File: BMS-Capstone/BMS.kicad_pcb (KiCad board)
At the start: 2 copper layers, 16 parts, among them IC1 MP2643, Q1 FODM121, Q2 FODM121

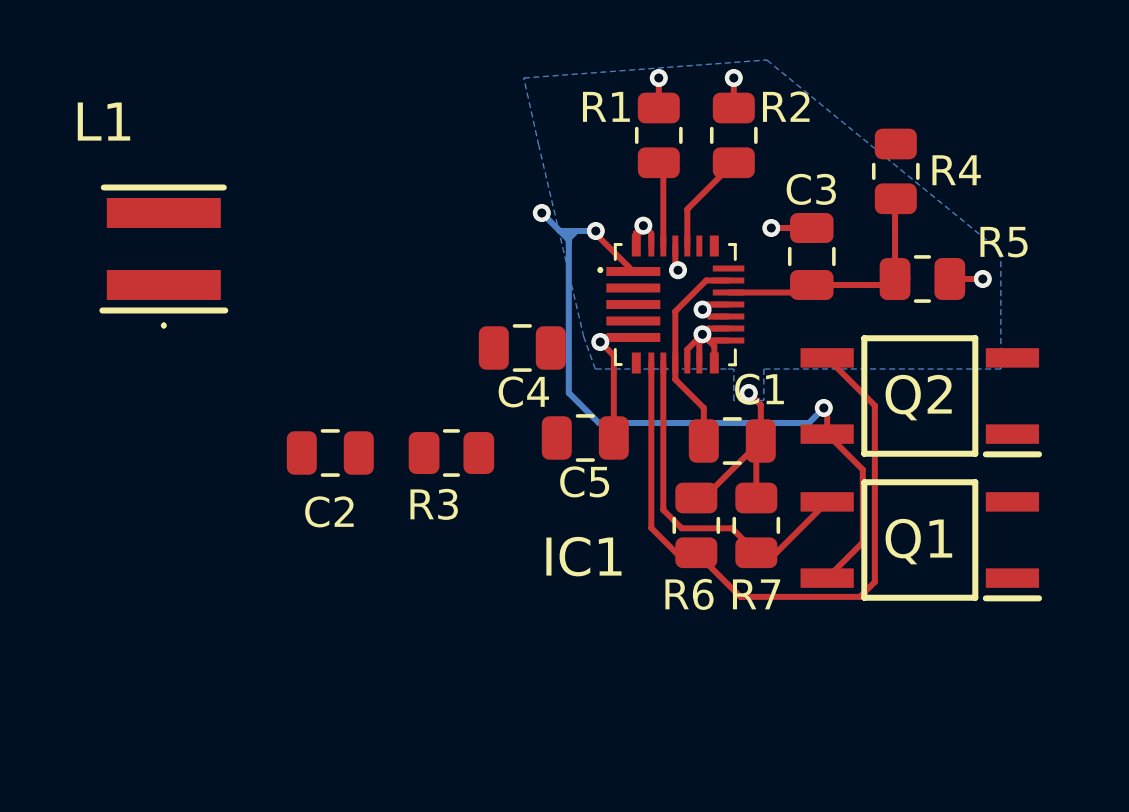
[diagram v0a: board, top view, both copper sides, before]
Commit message: Redid the whole thing
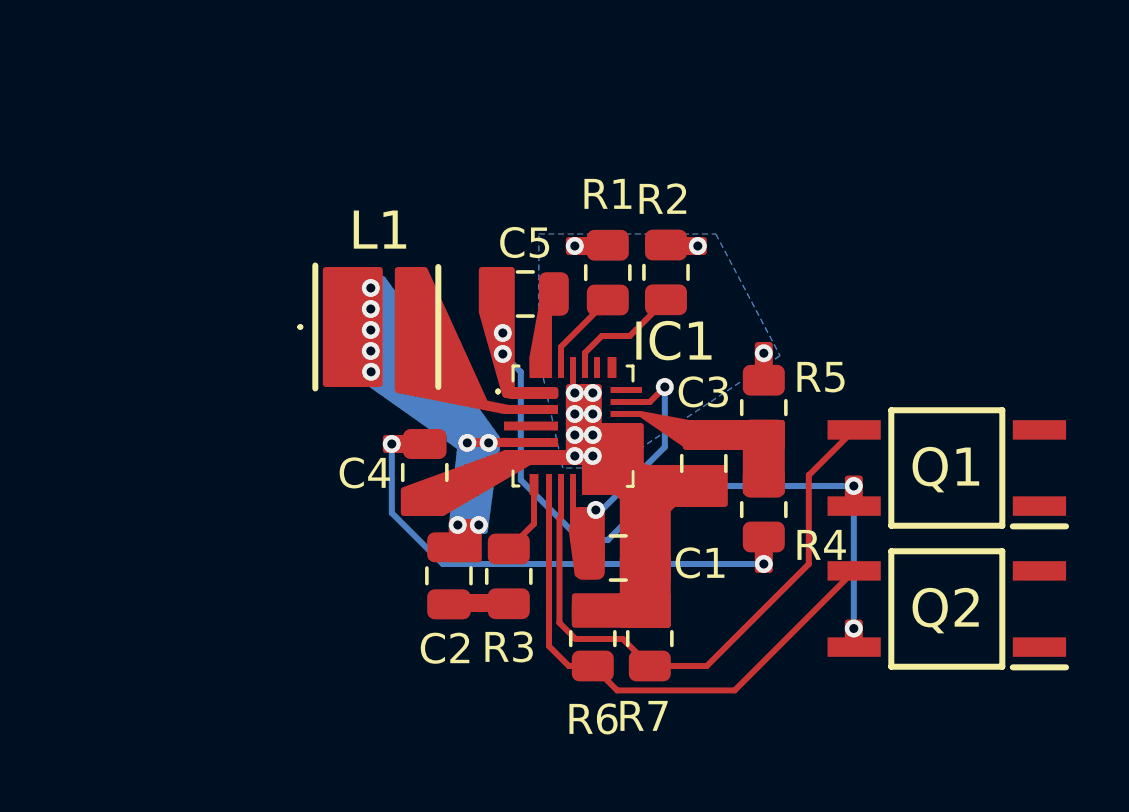
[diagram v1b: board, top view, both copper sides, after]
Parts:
- moved R4 12.1 mm to (158.5, 81.4), turned to 90 degrees
- moved C3 7.78 mm to (156.5, 79.8), turned to 90 degrees
- moved L1 7.56 mm to (145.6, 75.3), turned to 0 degrees
- moved Q2 7.16 mm to (164.6, 84.7)
- moved R5 6.81 mm to (158.5, 78.0), turned to 90 degrees
- moved C2 5.69 mm to (148.0, 83.6), turned to 90 degrees
- moved C1 5.45 mm to (153.7, 83.0)
- moved IC1 5.29 mm to (152.1, 78.6)
- moved C4 5.27 mm to (147.2, 80.2), turned to -90 degrees
- moved C5 5.20 mm to (150.6, 74.2)
- moved R7 5.18 mm to (154.7, 85.7)
- moved R6 5.11 mm to (152.8, 85.7)
- moved R2 5.10 mm to (155.2, 73.5)
- moved R1 4.88 mm to (153.3, 73.5)
- moved R3 4.54 mm to (150.0, 83.6), turned to 90 degrees
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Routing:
- net /BMS Board/1GND: track 25.4 -> 3.39 mm, vias 10 -> 11
- net /BMS Board/1Upper: track 0.35 -> 15.5 mm, vias 0 -> 2
- net Net-(IC1-CU_FB): track 8.67 -> 0.00 mm
- net Net-(IC1-MODE): track 11.9 -> 20.0 mm
- net Net-(IC1-EN): track 22.2 -> 17.8 mm
- net /BMS Board/1Lower: track 26.0 -> 22.6 mm, vias 3 -> 4
- net Net-(IC1-BST): track 0.00 -> 2.50 mm
- net /BMS Board/VCC1: track 6.92 -> 8.83 mm, vias 0 -> 2
- net Net-(IC1-LBC): track 3.42 -> 3.92 mm
- net Net-(IC1-SW): track 0.00 -> 0.09 mm, vias 0 -> 9
